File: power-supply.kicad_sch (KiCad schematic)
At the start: 20 parts, among them Q10 AO3401A, Q9 AO3401A, U8 TPS61230DRC, U9 LM3670MF

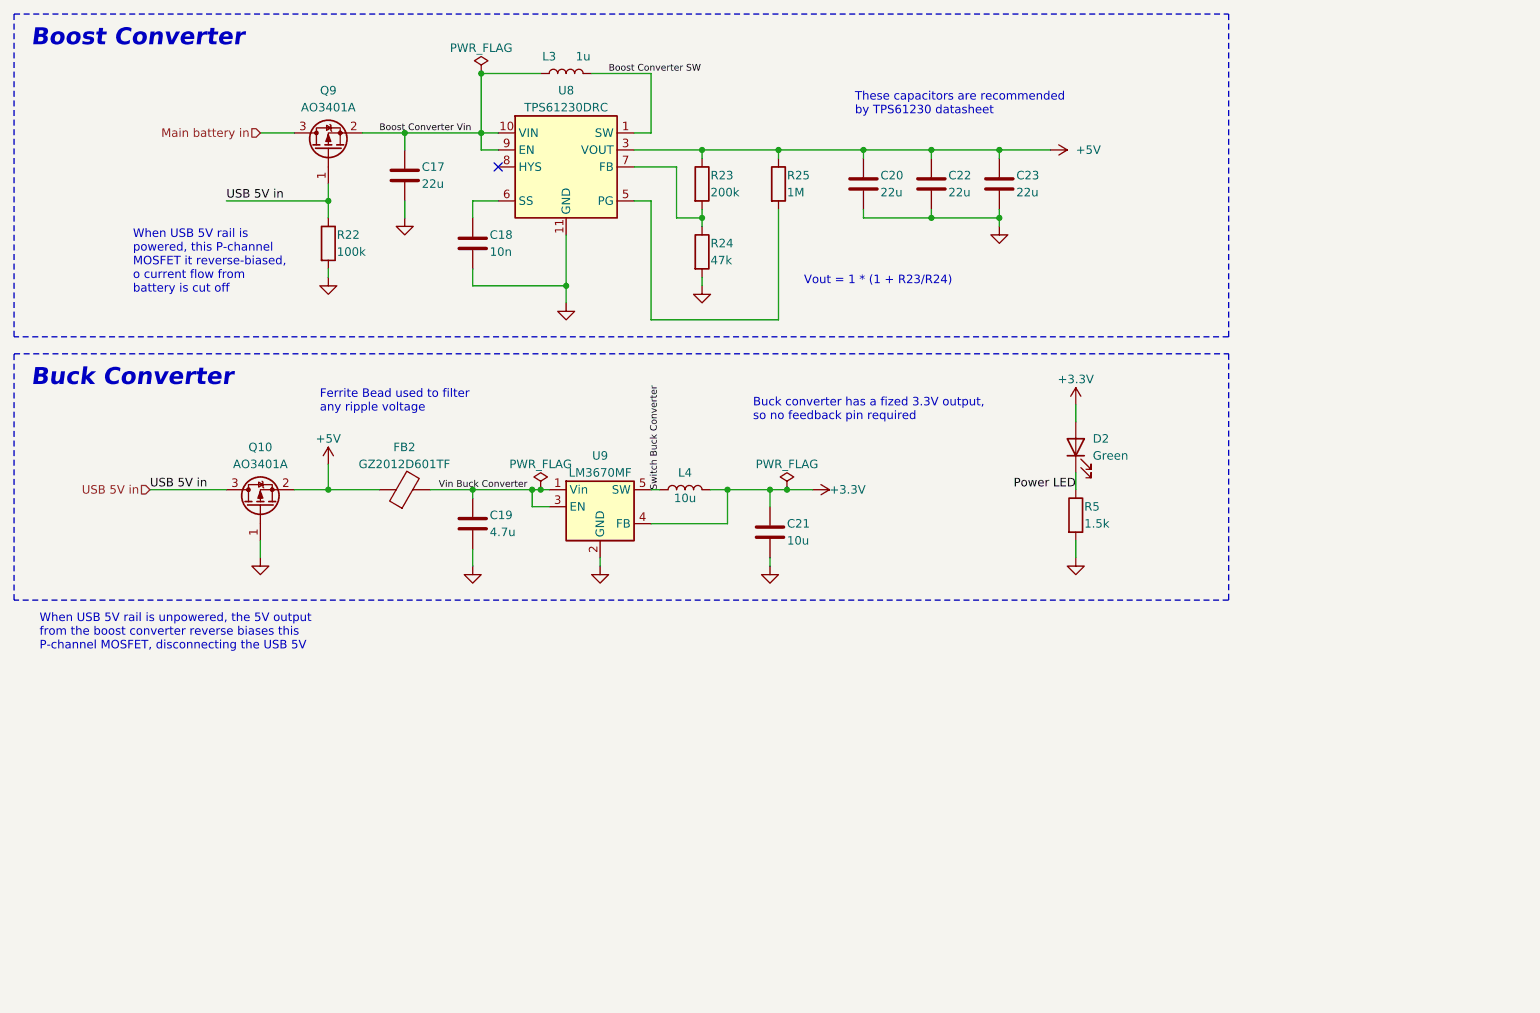
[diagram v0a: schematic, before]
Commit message: Started doing layout for v1.1
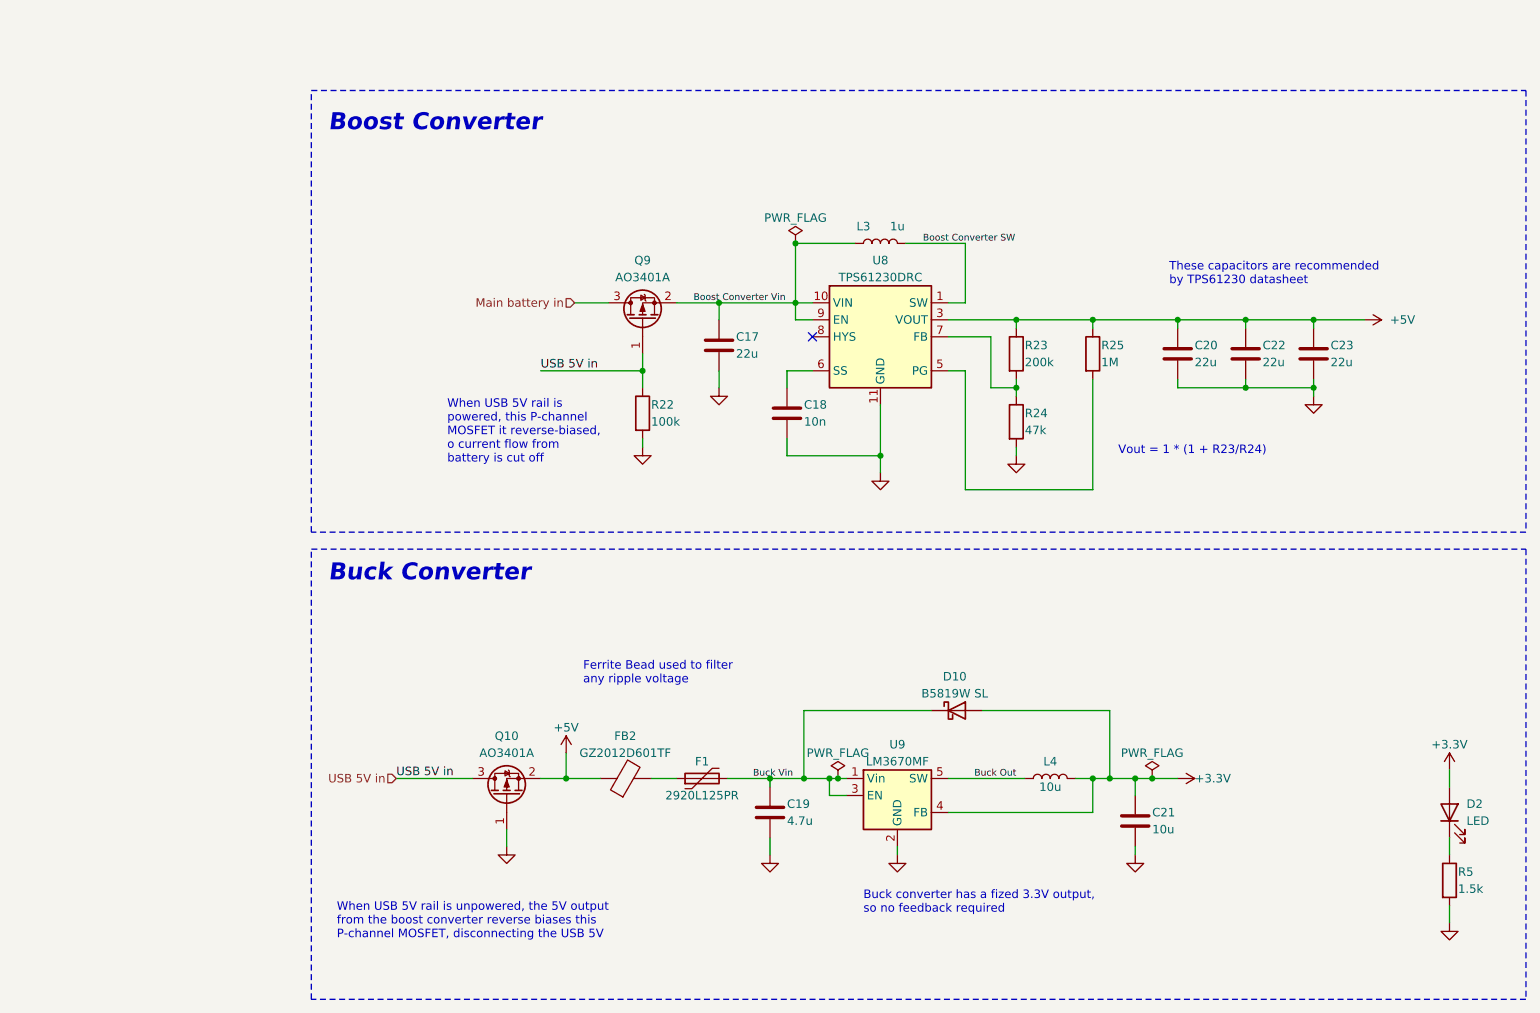
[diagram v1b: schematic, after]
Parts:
- added D10: B5819W SL, Diode_SMD:D_SOD-123, symbol Device:D_Schottky
- added F1: 2920L125PR, Fuse:Fuse_0805_2012Metric, symbol Device:Polyfuse
- D2: value Green -> LED; footprint LED_SMD:LED_0805_2012Metric -> LED_SMD:LED_0603_1608Metric
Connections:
- net +3.3V: now also D10.2 (A)
- net Power LED: no longer names the net of D2.1 (K), R5.1
- net Switch Buck Converter renamed Buck Out
- net Vin Buck Converter renamed Buck Vin
- net Buck Vin: now also D10.1 (K), F1.2; no longer FB2.2
- new net: F1.1, FB2.2
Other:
- note added: "Buck converter has a fized 3.3V output, so no feedback required"
- note removed: "Buck converter has a fized 3.3V output, so no feedback pin required"
- moved on the sheet: C17, C18, C19, C20, C21, C22, C23, D2, FB2, L3, L4, Q10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

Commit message: finished layout for v1.1
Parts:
- R5: footprint Resistor_SMD:R_0603_1608Metric -> Resistor_SMD:R_0402_1005Metric
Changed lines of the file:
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@@
       (effects (font (size 1.27 1.27)) (justify left))
     )
-    (property "Footprint" "Resistor_SMD:R_0603_1608Metric" (at 226.822 143.51 90)
+    (property "Footprint" "Resistor_SMD:R_0402_1005Metric" (at 226.822 143.51 90)
       (effects (font (size 1.27 1.27)) hide)
     )
